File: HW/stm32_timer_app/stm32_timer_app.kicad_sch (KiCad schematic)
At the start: 62 parts, among them J1 105164-0001, J2 61300411121, J3 61300411121, J4 691213710002, J5 691213710002, U1 RT9193-33GB, U2 MOC3041SM, U3 STM32F103C8T6, U4 MAX31865 AMPLIFIER, U5 MMBT2222A-7-F, Y1 ABLS-8.000MHZ-B2-T, Y2 ABS25-32.768KHZ-6-4-T

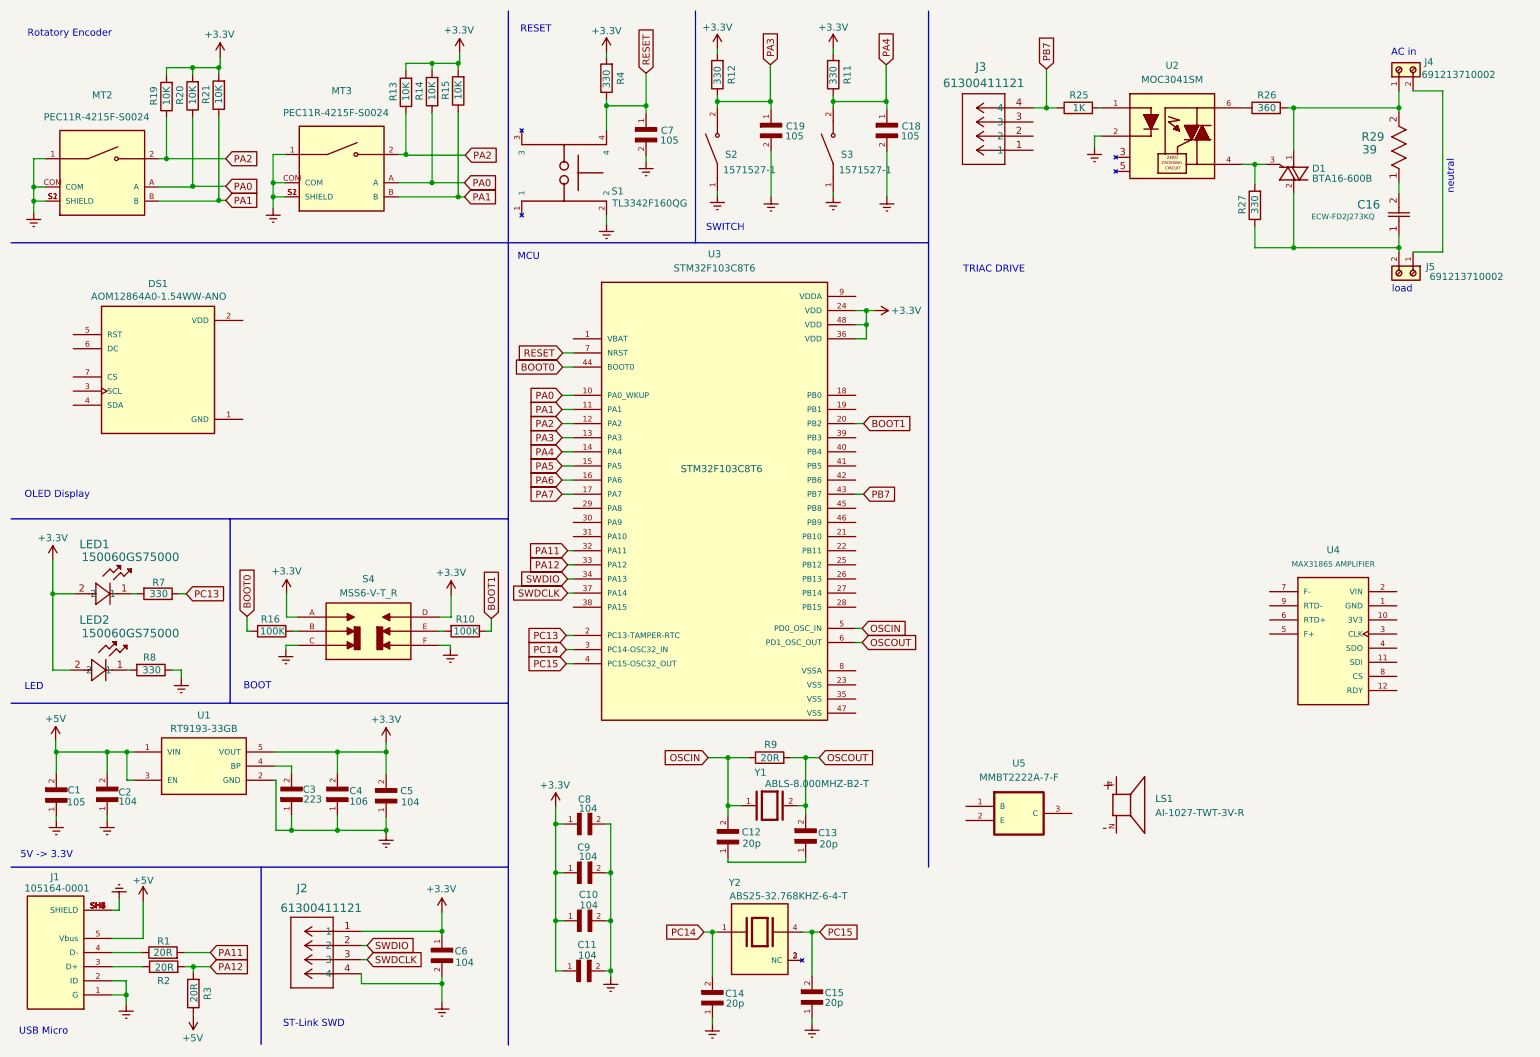
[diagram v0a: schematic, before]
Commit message: schematic
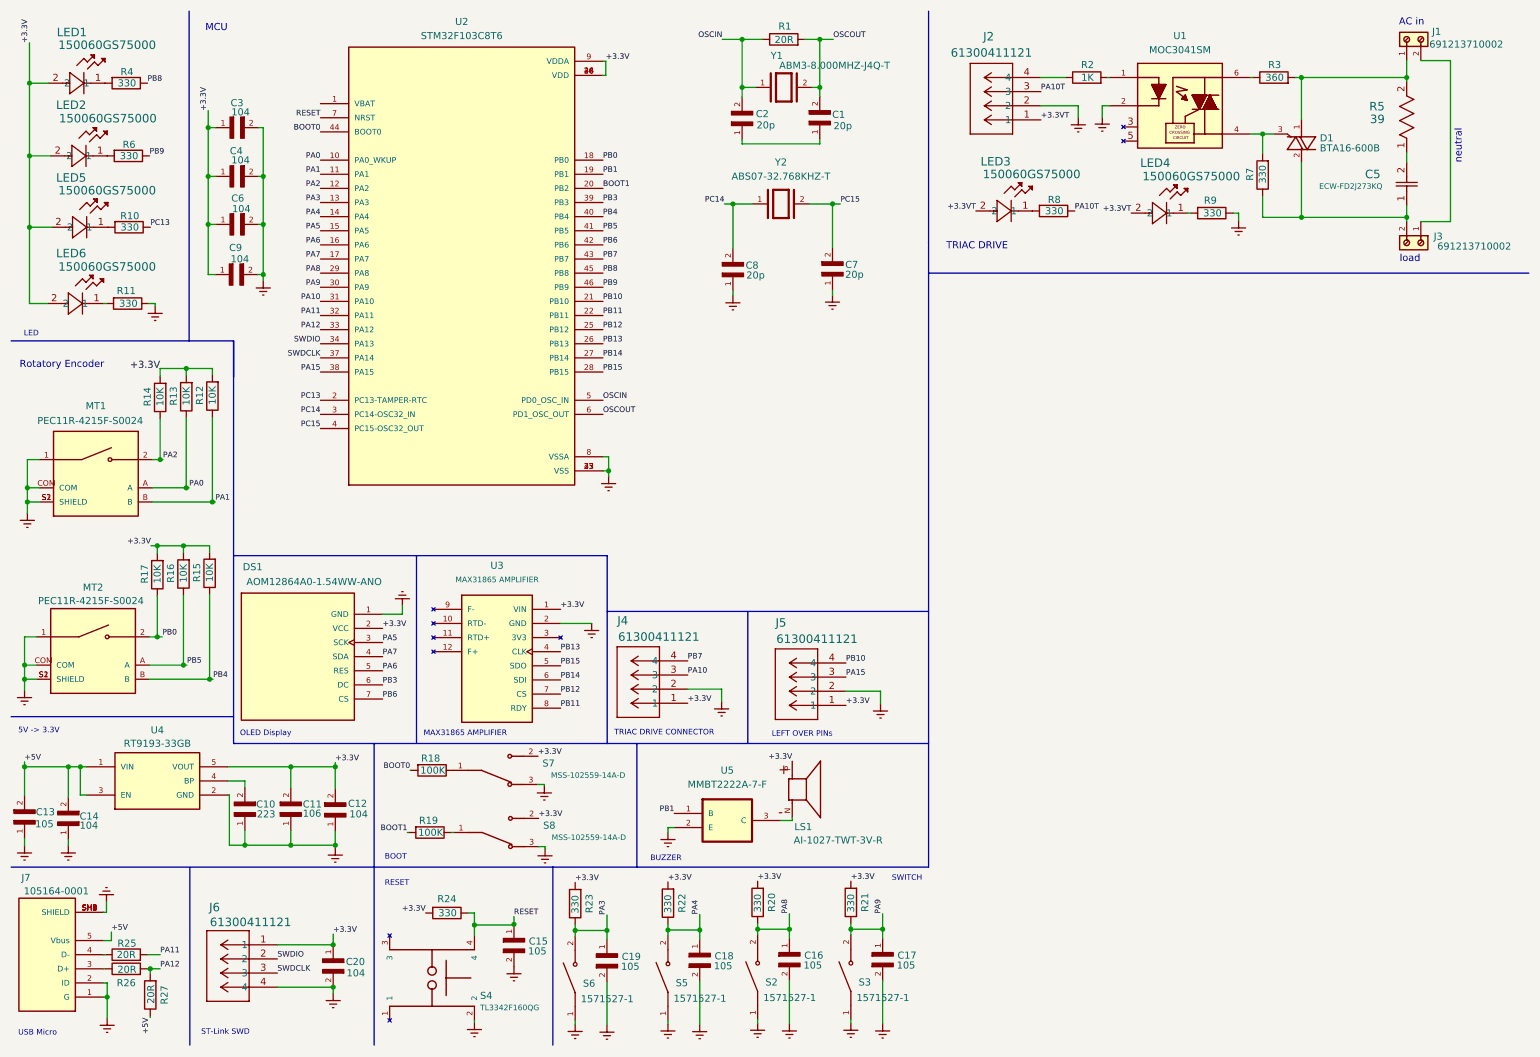
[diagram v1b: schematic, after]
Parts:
- removed R10: 100K, Resistor_SMD:R_0603_1608Metric, symbol Device:R
- removed R11: 330, Resistor_SMD:R_0603_1608Metric, symbol Device:R
- removed S4: MSS6-V-T_R, MSS6-V-T_R:SW_MSS6-V-T_R, symbol MSS6-V-T_R:MSS6-V-T_R
- removed U3: STM32F103C8T6, STM32F103C8T6:QFP50P900X900X160-48N, symbol STM32F103C8T6:STM32F103C8T6
- removed U4: MAX31865 AMPLIFIER, MAX31865:MAX31865, symbol MAX31865:MAX31865 AMPLIFIER
- removed Y1: ABLS-8.000MHZ-B2-T, ABLS-8.000MHZ-B2-T:XTAL_ABLS-8.000MHZ-B2-T, symbol ABLS-8.000MHZ-B2-T:ABLS-8.000MHZ-B2-T
- removed Y2: ABS25-32.768KHZ-6-4-T, ABS25-32.768KHZ-6-4-T:XTAL_ABS25-32.768KHZ-6-4-T, symbol ABS25-32.768KHZ-6-4-T:ABS25-32.768KHZ-6-4-T
- added C16, C17: 105, LD03ZD475MAB2A:CAPC1608X90, symbol LD03ZD475MAB2A:LD03ZD475MAB2A
- added J4, J5: 61300411121, 61300411121:CONN_61300411121_WRE, symbol 61300411121:61300411121
- added LED1, LED2: 150060GS75000, 150060GS75000:LED_150060GS75000_WRE, symbol 150060GS75000:150060GS75000
- added LED3, LED4: 150060GS75000, LED_150060GS75000_WRE, symbol 150060GS75000:150060GS75000
- added R19: 100K, Resistor_SMD:R_0603_1608Metric, symbol Device:R
- added R20, R21, R22, R4, R6, R8, R9: 330, Resistor_SMD:R_0603_1608Metric, symbol Device:R
- added S2, S5: 1571527-1, 1571527-1:SW_1571527-1, symbol 1571527-1:1571527-1
- added S7, S8: MSS-102559-14A-D, MSS-102559-14A-D:SW_MSS-102559-14A-D, symbol MSS-102559-14A-D:MSS-102559-14A-D
- added U2: STM32F103C8T6, STM32F103C8T6:QFP50P900X900X160-48N, symbol STM32F103C8T6:STM32F103C8T6
- added U3: MAX31865 AMPLIFIER, MAX31865:MAX31865, symbol MAX31865:MAX31865 AMPLIFIER
- added Y1: ABM3-8.000MHZ-J4Q-T, ABM3_8_000MHZ_J4Q_T:XTAL_ABM3-8.000MHZ-J4Q-T, symbol ABM3-8.000MHZ-J4Q-T:ABM3-8.000MHZ-J4Q-T
- added Y2: ABS07-32.768KHZ-T, ABS07-32.768KHZ-T:XTAL_ABS07-32.768KHZ-T, symbol ABS07-32.768KHZ-T:ABS07-32.768KHZ-T
- LED5: renamed from LED1; footprint LED_150060GS75000_WRE -> 150060GS75000:LED_150060GS75000_WRE
- LED6: renamed from LED2; footprint LED_150060GS75000_WRE -> 150060GS75000:LED_150060GS75000_WRE
- renumbered C13 to C1, C3 to C10, C4 to C11, C5 to C12, C1 to C13, C2 to C14, C7 to C15, C12 to C2, C6 to C20, C8 to C3, C9 to C4, C16 to C5, C10 to C6, C15 to C7, C14 to C8, C11 to C9, J4 to J1, J3 to J2, J5 to J3, J2 to J6, J1 to J7, MT3 to MT1, R9 to R1, R7 to R10, R8 to R11, R15 to R12, R14 to R13, R13 to R14, R21 to R15, R20 to R16, R19 to R17, R16 to R18, R25 to R2, R12 to R23, R4 to R24, R1 to R25, R2 to R26, R3 to R27, R26 to R3, R29 to R5, R27 to R7, S1 to S4, S2 to S6, U2 to U1, U1 to U4
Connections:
- net +3.3V: now also DS1.2 (VCC), LS1.P, J4.1, J5.1, LED1.2, LED2.2, R20.2, R21.2, R22.2, S7.2, S8.2, U2.24 (VDD), U2.36 (VDD), U2.48 (VDD), U2.9 (VDDA), U3.1 (VIN)
- net BOOT0: now also U2.44 (BOOT0)
- net BOOT1: now also R19.2, U2.20 (PB2)
- net OSCIN: now also U2.5 (PD0_OSC_IN), Y1.1
- net OSCOUT: now also U2.6 (PD1_OSC_OUT), Y1.2
- net PA0: now also U2.10 (PA0_WKUP); no longer MT2.A, R16.1
- net PA1: now also U2.11 (PA1); no longer MT2.B, R15.1
- net PA11: now also U2.32 (PA11)
- net PA12: now also U2.33 (PA12)
- net PA2: now also U2.12 (PA2); no longer MT2.2, R17.1
- net PA3: now also U2.13 (PA3)
- net PA4: now also R22.1, S5.2, S5.4, U2.14 (PA4); no longer S3.2, S3.4
- net PA5: now also DS1.3 (SCK), U2.15 (PA5)
- net PA6: now also DS1.5 (RES), U2.16 (PA6)
- net PA7: now also DS1.4 (SDA), U2.17 (PA7)
- net PB7: now also J4.4, U2.43 (PB7); no longer J2.4, R2.1
- net PC13: now also U2.2 (PC13-TAMPER-RTC)
- net PC14: now also U2.3 (PC14-OSC32_IN), Y2.1
- net PC15: now also U2.4 (PC15-OSC32_OUT), Y2.2
- net RESET: now also U2.7 (NRST)
- net SWDCLK: now also U2.37 (PA14)
- net SWDIO: now also U2.34 (PA13)
- net PB1: now reaches U5.1 (B)
- net PB1: now also U2.19 (PB1)
- net at U5.3 (C): now also LS1.N
- net +3.3VT: now reaches J2.1
- net +3.3VT: now also LED3.2, LED4.2
- net PA10T: now reaches J2.3
- net PA10T: now also R8.1
- net PB3: now reaches DS1.6 (DC)
- net PB3: now also U2.39 (PB3)
- net PB6: now reaches DS1.7 (CS)
- net PB6: now also U2.42 (PB6)
- net at R18.1: now also S7.1
- new net: J2.4, R2.1
- new net: LED1.1, R4.2
- new net: LED2.1, R6.2
- new net: LED4.1, R9.2
- new net: S5.1, S5.3
- new net: R19.1, S8.1
- new net: LED3.1, R8.2
- new net: S2.1, S2.3
- new net: U2.23 (VSS), U2.35 (VSS), U2.47 (VSS), U2.8 (VSSA)
- new net PA10: J4.3, U2.31 (PA10)
- new net PA15: J5.3, U2.38 (PA15)
- new net PA8: C16.1, R20.1, S2.2, S2.4, U2.29 (PA8)
- new net PA9: C17.1, R21.1, S3.2, S3.4, U2.30 (PA9)
- new net PB0: MT2.2, R17.1, U2.18 (PB0)
- new net PB10: J5.4, U2.21 (PB10)
- new net PB11: U2.22 (PB11), U3.8 (RDY)
- new net PB12: U2.25 (PB12), U3.7 (CS)
- new net PB13: U2.26 (PB13), U3.4 (CLK)
- new net PB14: U2.27 (PB14), U3.6 (SDI)
- new net PB15: U2.28 (PB15), U3.5 (SDO)
- new net PB4: MT2.B, R15.1, U2.40 (PB4)
- new net PB5: MT2.A, R16.1, U2.41 (PB5)
- new net PB8: R4.1, U2.45 (PB8)
- new net PB9: R6.1, U2.46 (PB9)
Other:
- note added: "BUZZER"
- note added: "LEFT OVER PINs"
- note added: "MAX31865 AMPLIFIER"
- note added: "TRIAC DRIVE CONNECTOR"
- moved on the sheet: C1, C10, C11, C12, C13, C14, C15, C19, C2, C20, C3, C4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
